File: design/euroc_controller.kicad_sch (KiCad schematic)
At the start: 63 parts, among them J1 xt30, J2 jst_sh 4, J4 jst_sh 4, J5 jst_sh 4, J6 SMA, J8 USB_C_Receptacle_USB2.0, J9 jst_sh 4, Q1 MMBT3904, U1 TPSM5601R5, U12 STM32L562CETx, U2 USBLC6-2SC6, U3 LSM6DSO32, U4 MS5611-01BA, U5 SN65HVD232, U6 W25Q128JVS, U7 RFM69W, U8 L86, Y1 48MHz

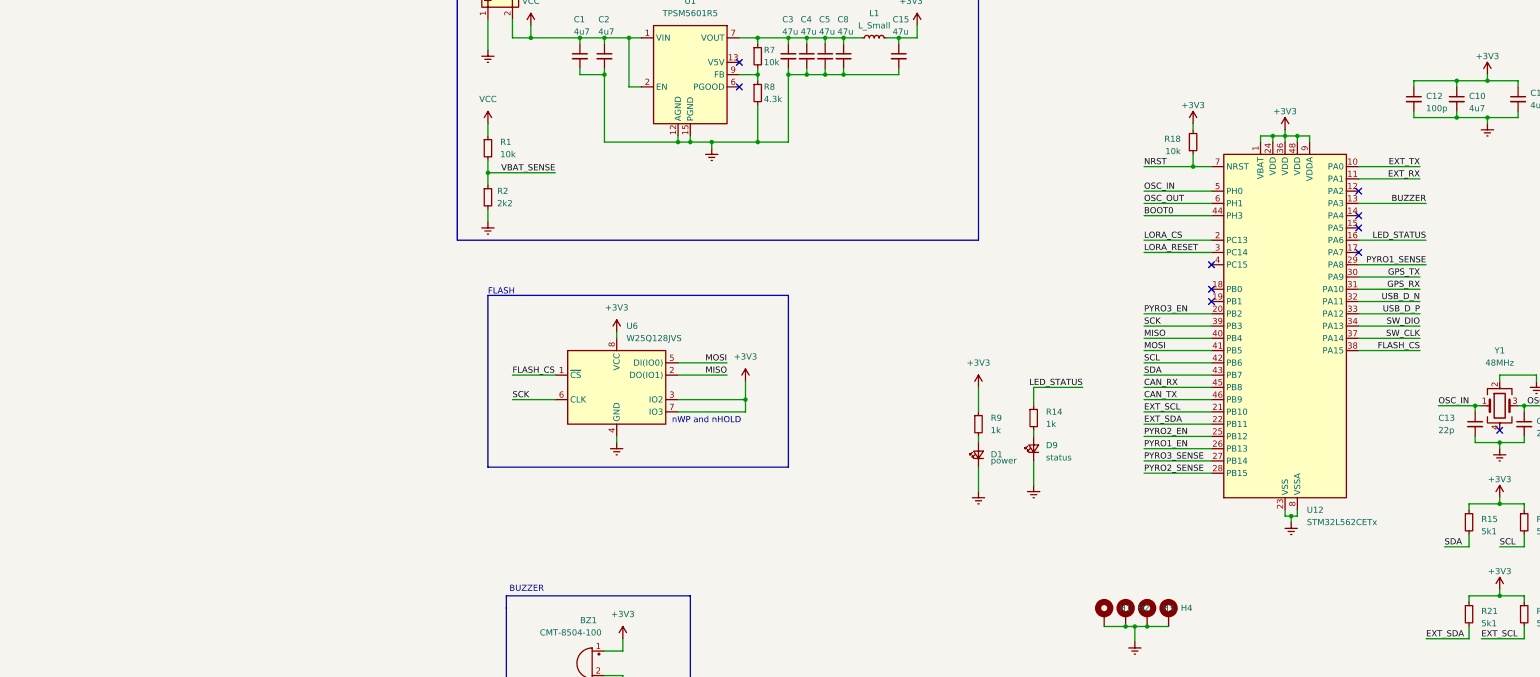
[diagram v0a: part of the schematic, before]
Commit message: oof new umc (st32u5)
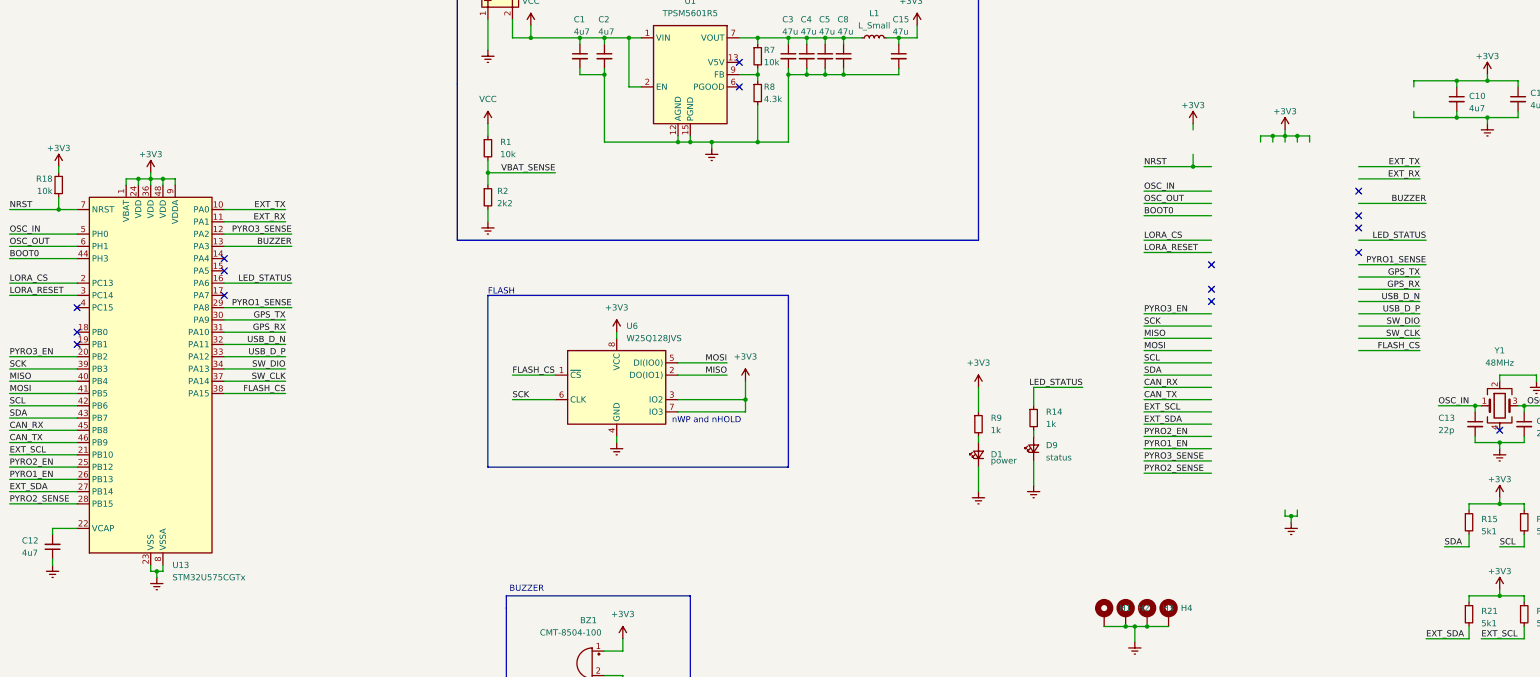
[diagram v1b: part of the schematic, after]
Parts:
- removed U12: STM32L562CETx, Package_QFP:LQFP-48_7x7mm_P0.5mm, symbol MCU_ST_STM32L5:STM32L562CETx
- added U13: STM32U575CGTx, Package_QFP:LQFP-48_7x7mm_P0.5mm, symbol MCU_ST_STM32U5:STM32U575CGTx
- C12: value 100p -> 4u7
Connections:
- net +3V3: now also U13.1 (VBAT), U13.24 (VDD), U13.36 (VDD), U13.48 (VDD), U13.9 (VDDA); no longer C12.1
- net BOOT0: now also U13.44 (PH3)
- net BUZZER: now also U13.13 (PA3)
- net CAN_RX: now also U13.45 (PB8)
- net CAN_TX: now also U13.46 (PB9)
- net EXT_RX: now also U13.11 (PA1)
- net EXT_SCL: now also U13.21 (PB10)
- net EXT_SDA: now also U13.27 (PB14)
- net EXT_TX: now also U13.10 (PA0)
- net Earth: now also C12.1, U13.23 (VSS), U13.35 (VSS), U13.47 (VSS), U13.8 (VSSA); no longer C12.2
- net FLASH_CS: now also U13.38 (PA15)
- net GPS_RX: now also U13.31 (PA10)
- net GPS_TX: now also U13.30 (PA9)
- net LED_STATUS: now also U13.16 (PA6)
- net LORA_CS: now also U13.2 (PC13)
- net LORA_RESET: now also U13.3 (PC14)
- net MISO: now also U13.40 (PB4)
- net MOSI: now also U13.41 (PB5)
- net NRST: now also U13.7 (NRST)
- net OSC_IN: now also U13.5 (PH0)
- net OSC_OUT: now also U13.6 (PH1)
- net PYRO1_EN: now also U13.26 (PB13)
- net PYRO1_SENSE: now also U13.29 (PA8)
- net PYRO2_EN: now also U13.25 (PB12)
- net PYRO2_SENSE: now also U13.28 (PB15)
- net PYRO3_EN: now also U13.20 (PB2)
- net PYRO3_SENSE: now also U13.12 (PA2)
- net SCK: now also U13.39 (PB3)
- net SCL: now also U13.42 (PB6)
- net SDA: now also U13.43 (PB7)
- net SW_CLK: now also U13.37 (PA14)
- net SW_DIO: now also U13.34 (PA13)
- net USB_D_N: now also U13.32 (PA11)
- net USB_D_P: now also U13.33 (PA12)
- new net: C12.2, U13.22 (VCAP)
- no-connect marks 25 -> 31
